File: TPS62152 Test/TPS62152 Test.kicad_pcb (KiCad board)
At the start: 2 copper layers, 29.4 x 23 mm, 17 parts, among them J1 Conn_01x02_Pin, J2 Conn_01x02_Pin, J3 Conn_01x02_Pin, J4 Conn_01x02_Socket, U1 TPS62152RGTR

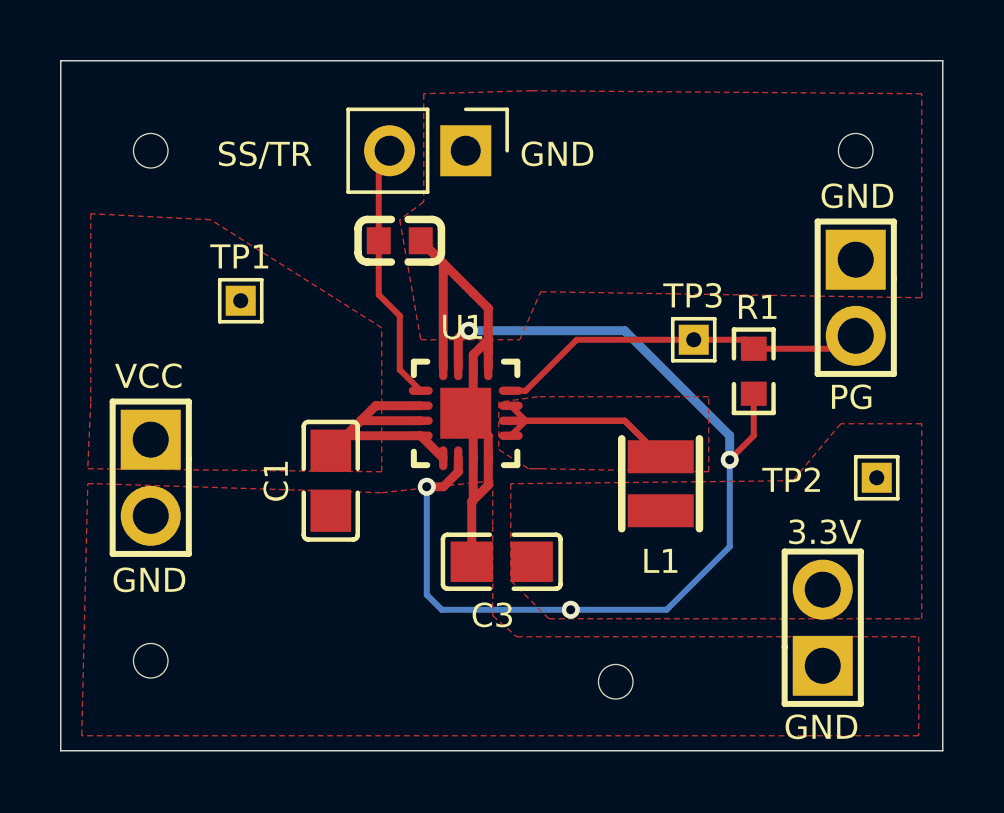
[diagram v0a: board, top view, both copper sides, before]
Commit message: tidy up
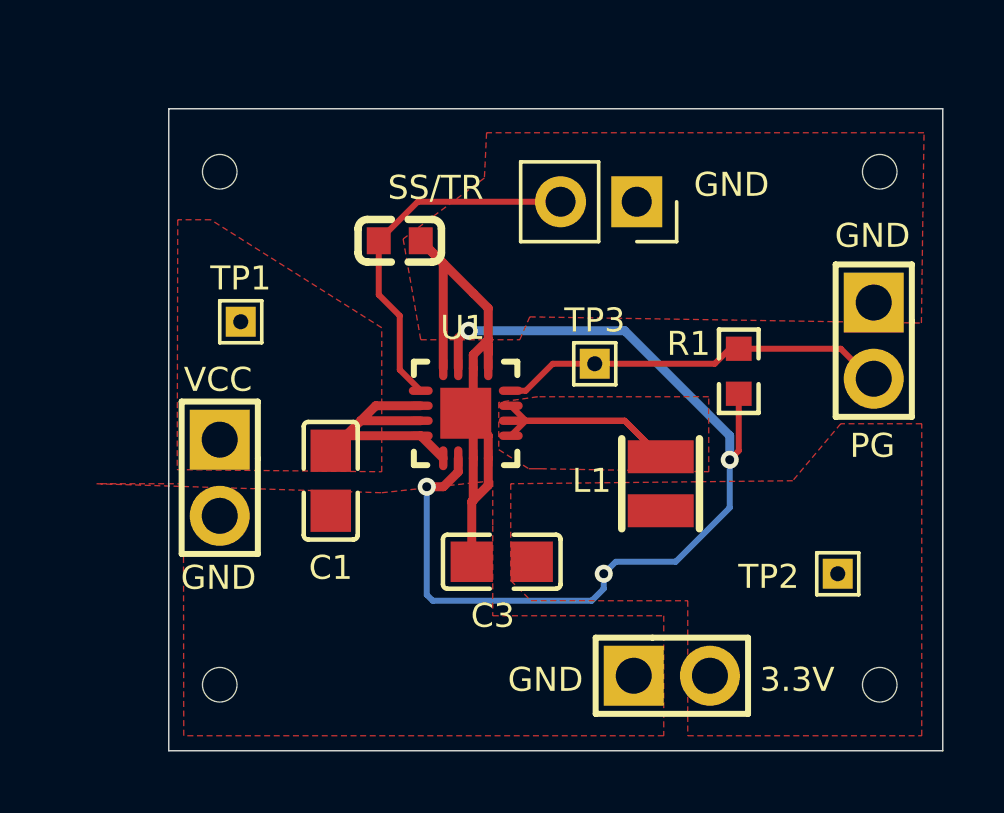
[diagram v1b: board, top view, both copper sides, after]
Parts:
- removed H1, H2, H3, H4: MountingHole, MountingHole:ToolingHole_1.152mm
- added REF**: ToolingHole_1.152mm, MountingHole:ToolingHole_1.152mm, F.Cu at (183.3, 123.8)
- added REF**: ToolingHole_1.152mm, MountingHole:ToolingHole_1.152mm, F.Cu at (183.3, 106.7)
- added REF**: ToolingHole_1.152mm, MountingHole:ToolingHole_1.152mm, F.Cu at (161.3, 123.8)
- added REF**: ToolingHole_1.152mm, MountingHole:ToolingHole_1.152mm, F.Cu at (161.3, 106.7)
- J4: footprint Connector_PinHeader_2.54mm:PinHeader_1x02_P2.54mm_Vertical -> Connector_PinSocket_2.54mm:PinSocket_1x02_P2.54mm_Vertical
- moved J4 5.95 mm to (175.2, 107.7)
- moved J2 5.28 mm to (176.4, 123.5), turned to 0 degrees
- moved TP2 3.45 mm to (181.9, 120.1)
- moved TP3 3.40 mm to (173.8, 113.1)
- moved J1 2.30 mm to (161.3, 116.9)
- moved J3 1.55 mm to (183.1, 112.3)
- moved TP1 0.70 mm to (162.0, 111.7)
- moved R1 0.50 mm to (178.6, 113.3)
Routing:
- net /SSTR: track 8.73 -> 12.2 mm
- net +3.3V: track 34.3 -> 33.4 mm
- net /POWER_GOOD: track 12.5 -> 13.1 mm
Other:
- board size 29.4 x 23 mm -> 25.8 x 21.4 mm
